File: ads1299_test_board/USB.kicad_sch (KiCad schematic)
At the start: 4 parts, among them P1 USB_C_Plug_USB2.0, SW3 SW_SPDT, U7 TPD4E05U06DQA

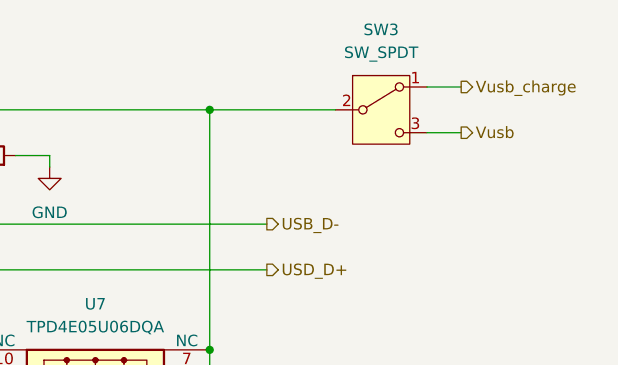
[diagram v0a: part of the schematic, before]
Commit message: PCB design charger and power supply
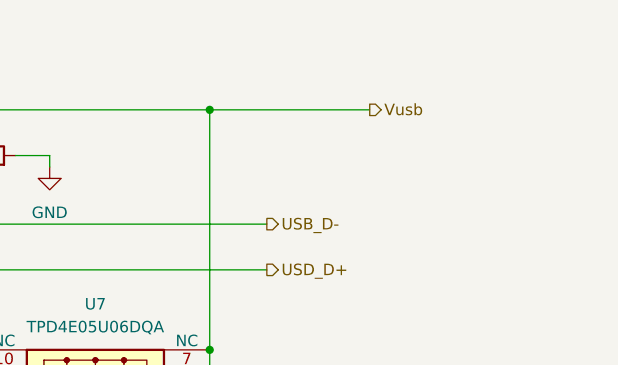
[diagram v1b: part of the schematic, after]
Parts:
- removed SW3: SW_SPDT, Button_Switch_THT:SW_Slide_SPDT_Straight_CK_OS102011MS2Q, symbol Switch:SW_SPDT
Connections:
- net Vbus is gone; now on net Vusb: P1.A4 (VBUS), P1.A9 (VBUS), P1.B4 (VBUS), P1.B9 (VBUS), U7.4 (D2+), U7.7 (NC)
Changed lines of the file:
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@@
-	(wire
-		(pts
-			(xy 184.15 78.74) (xy 187.96 78.74)
-		)
-		(stroke
-			(width 0)
-			(type default)
-		)
-	)
 	(wire
 		(pts
@@
 	(wire
 		(pts
-			(xy 160.02 76.2) (xy 173.99 76.2)
+			(xy 160.02 76.2) (xy 177.8 76.2)
 		)
 		(stroke
@@
 		(pts
 			(xy 130.81 93.98) (xy 166.37 93.98)
-		)
-		(stroke
-			(width 0)
-			(type default)
-		)
-	)
-	(wire
-		(pts
-			(xy 184.15 73.66) (xy 187.96 73.66)
 		)
 		(stroke
@@
 			)
 			(justify left bottom)
-		)
-	)
-	(hierarchical_label "Vusb_charge"
-		(shape output)
-		(at 187.96 73.66 0)
-		(effects
-			(font
-				(size 1.27 1.27)
-			)
-			(justify left)
 		)
 	)
@@
 	(hierarchical_label "Vusb"
 		(shape output)
-		(at 187.96 78.74 0)
+		(at 177.8 76.2 0)
 		(effects
 			(font
@@
 					(unit 1)
 				)
-			)
-		)
-	)
-	(symbol
-		(lib_id "Switch:SW_SPDT")
-		(at 179.07 76.2 0)
-		(unit 1)
-		(body_style 1)
-		(exclude_from_sim no)
-		(in_bom yes)
-		(on_board yes)
-		(in_pos_files yes)
-		(dnp no)
-		(fields_autoplaced yes)
-		(property "Reference" "SW3"
-			(at 179.07 67.31 0)
-			(show_name no)
-			(do_not_autoplace no)
-			(effects
-				(font
-					(size 1.27 1.27)
-				)
-			)
-		)
-		(property "Value" "SW_SPDT"
-			(at 179.07 69.85 0)
-			(show_name no)
-			(do_not_autoplace no)
-			(effects
-				(font
-					(size 1.27 1.27)
-				)
-			)
-		)
-		(property "Footprint" "Button_Switch_THT:SW_Slide_SPDT_Straight_CK_OS102011MS2Q"
-			(at 179.07 76.2 0)
-			(hide yes)
-			(show_name no)
-			(do_not_autoplace no)
-			(effects
-				(font
-					(size 1.27 1.27)
-				)
-			)
-		)
-		(property "Datasheet" ""
-			(at 179.07 83.82 0)
-			(hide yes)
-			(show_name no)
-			(do_not_autoplace no)
-			(effects
-				(font
-					(size 1.27 1.27)
-				)
-			)
-		)
-		(property "Description" "MFS101D-10-Z"
-			(at 179.07 76.2 0)
-			(hide yes)
-			(show_name no)
-			(do_not_autoplace no)
-			(effects
-				(font
-					(size 1.27 1.27)
-				)
-			)
-		)
-		(pin "1"
-		)
-		(pin "2"
-		)
-		(pin "3"
-		)
-		(instances
-			(project "ads1299_test_board"
-				(path "/97f9a33a-d3bd-406a-9672-b92babffe6b5/6847a2d3-404c-4489-885a-3855f072c603"
-					(reference "SW3")
-					(unit 1)
-				)
